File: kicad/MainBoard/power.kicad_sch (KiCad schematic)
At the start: 72 parts, among them J16 Conn_01x02_Female, J20 USB_C_Receptacle, SW1 SW_SPDT, U13 BQ27441-G1, U14 HY2111-GB, U15 FS8205A, U17 TPS61088, U2 BQ25601, U26 SN74LVC1G3157DCKR, U27 SN74LVC1G3157DCKR

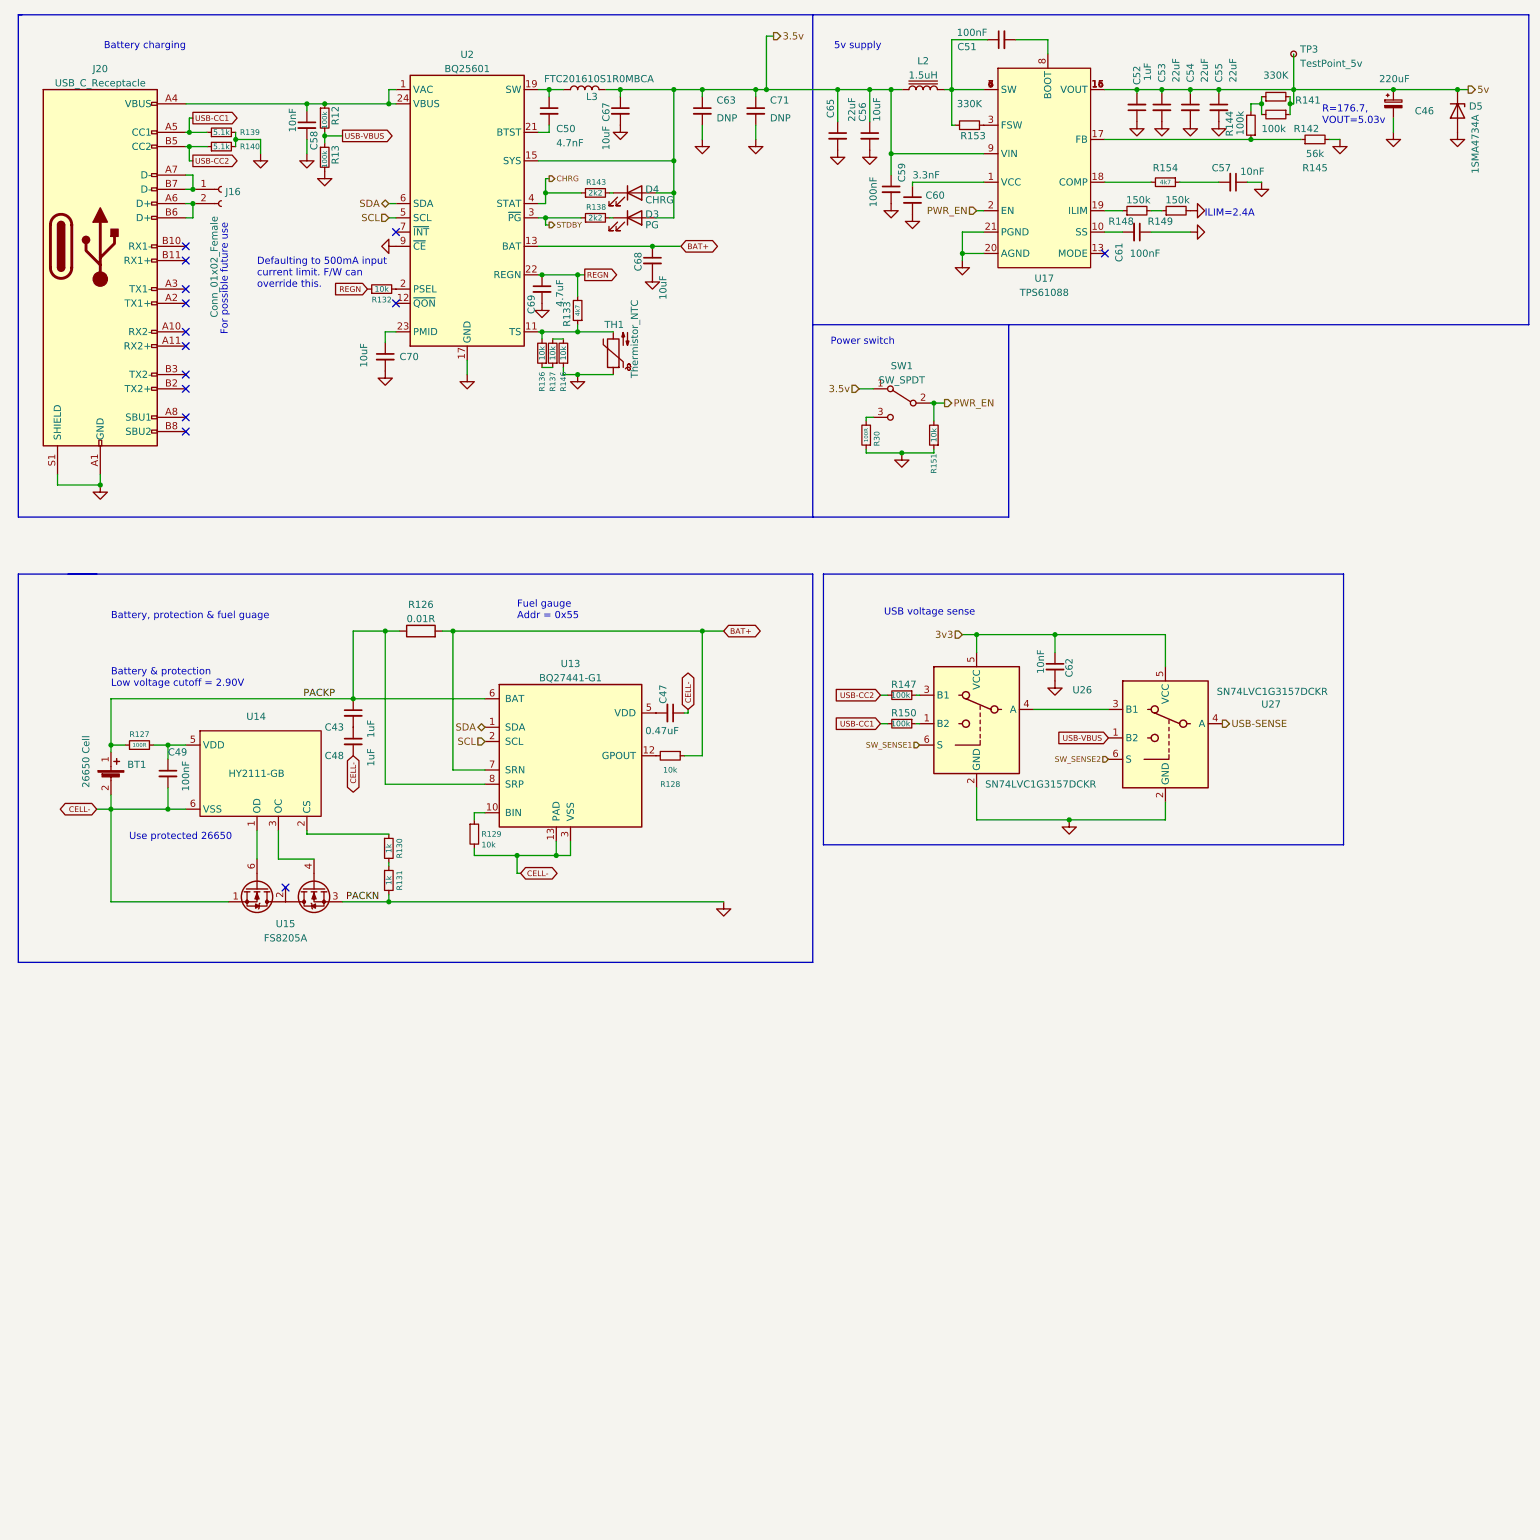
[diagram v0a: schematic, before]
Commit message: v2.5 schematic + PCB changes
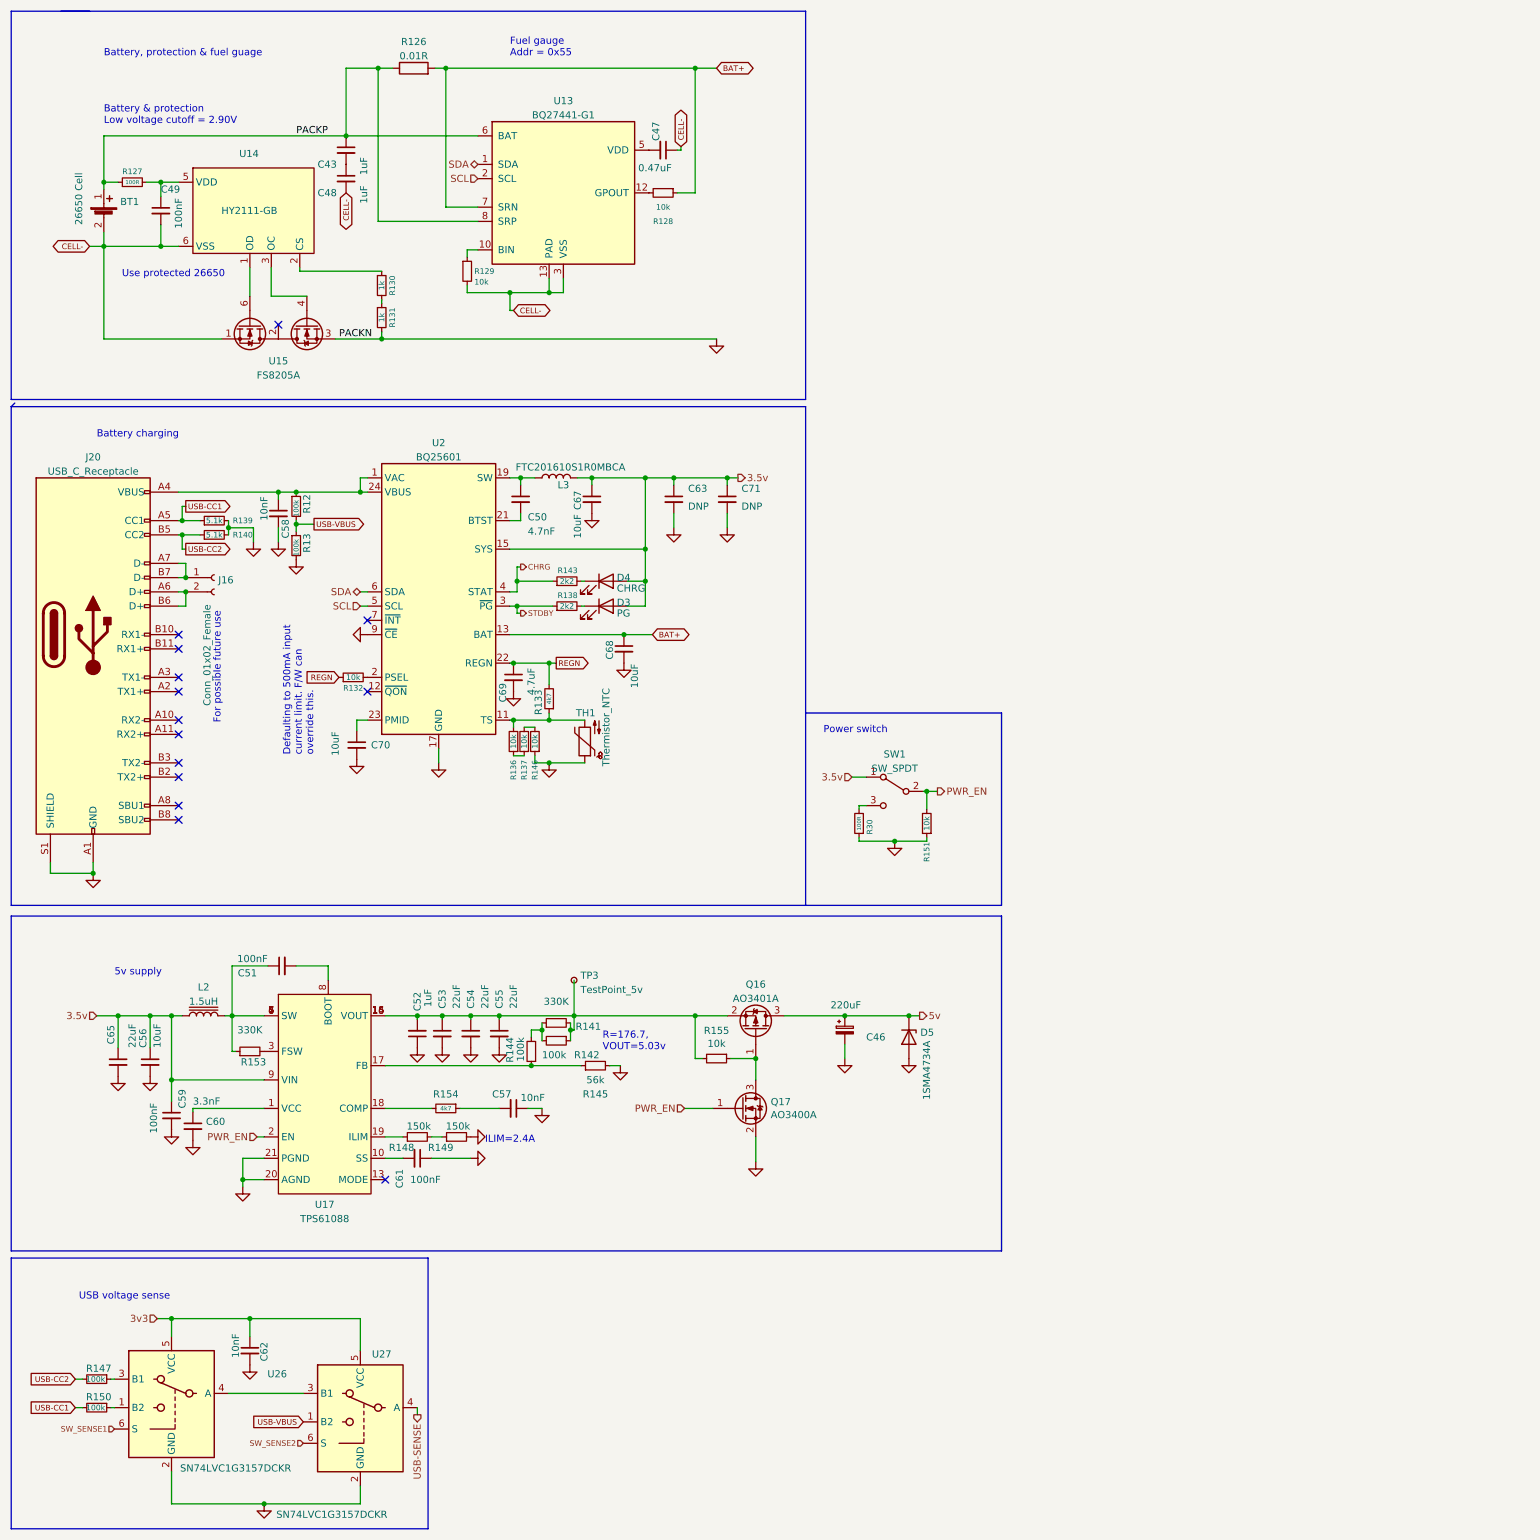
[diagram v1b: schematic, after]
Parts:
- added Q16: AO3401A, Package_TO_SOT_SMD:SOT-23_Handsoldering, symbol Transistor_FET:AO3401A
- added Q17: AO3400A, Package_TO_SOT_SMD:SOT-23_Handsoldering, symbol Device:Q_NMOS_GSD
- added R155: 10k, Resistor_SMD:R_0603_1608Metric_Pad0.98x0.95mm_HandSolder, symbol Device:R_Small
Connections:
- net 5v: now also Q16.3 (D); no longer C52.2, C53.1, C54.1, C55.1, R141.2, R142.1, TP3.1, U17.14 (VOUT), U17.15 (VOUT), U17.16 (VOUT)
- net GND: now also Q17.2 (S)
- net PWR_EN: now also Q17.1 (G)
- new net: C52.2, C53.1, C54.1, C55.1, Q16.2 (S), R141.2, R142.1, R155.2, TP3.1, U17.14 (VOUT), U17.15 (VOUT), U17.16 (VOUT)
- new net: Q16.1 (G), Q17.3 (D), R155.1
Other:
- company: (none) -> CrashOverride85
- title: (none) -> ZC95 MKII
- moved on the sheet: BT1, C43, C46, C47, C48, C49, C50, C51, C52, C53, C54, C55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
